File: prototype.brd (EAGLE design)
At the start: 100 x 80 mm, 15 parts

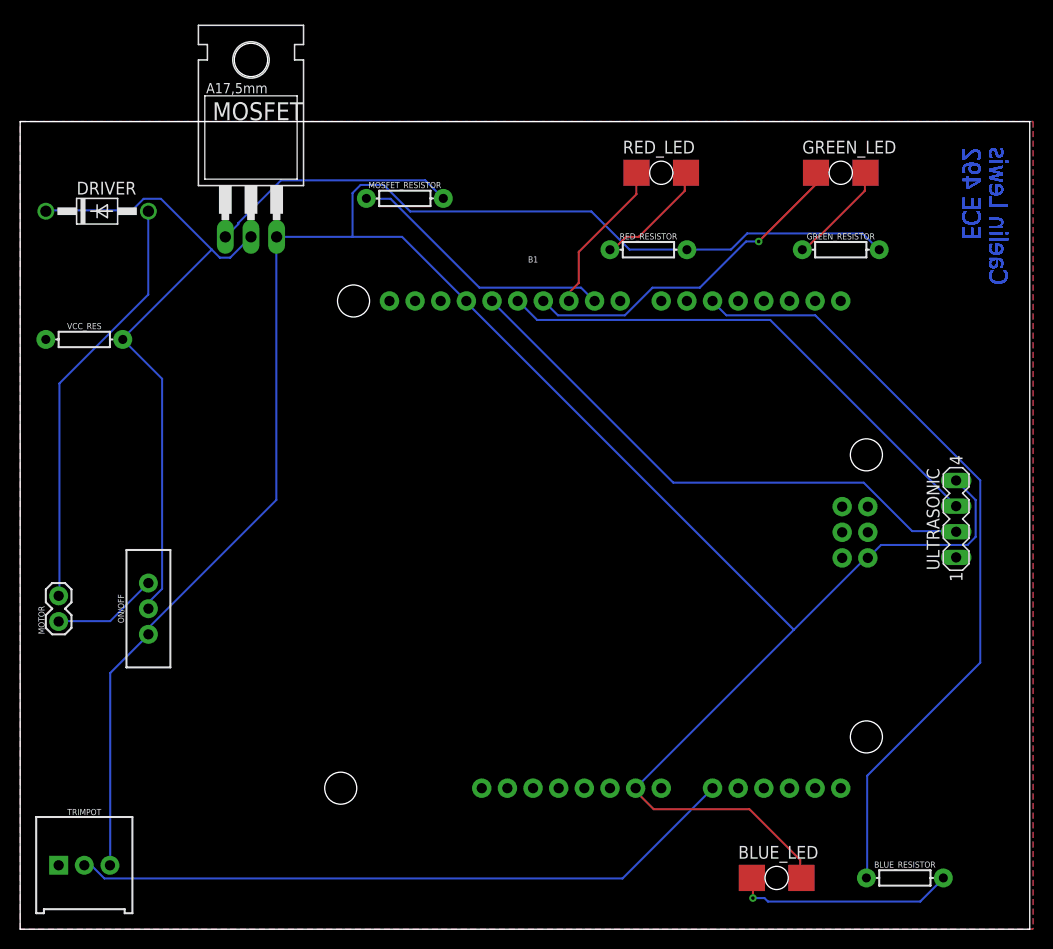
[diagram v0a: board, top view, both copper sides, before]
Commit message: Final Draft of board
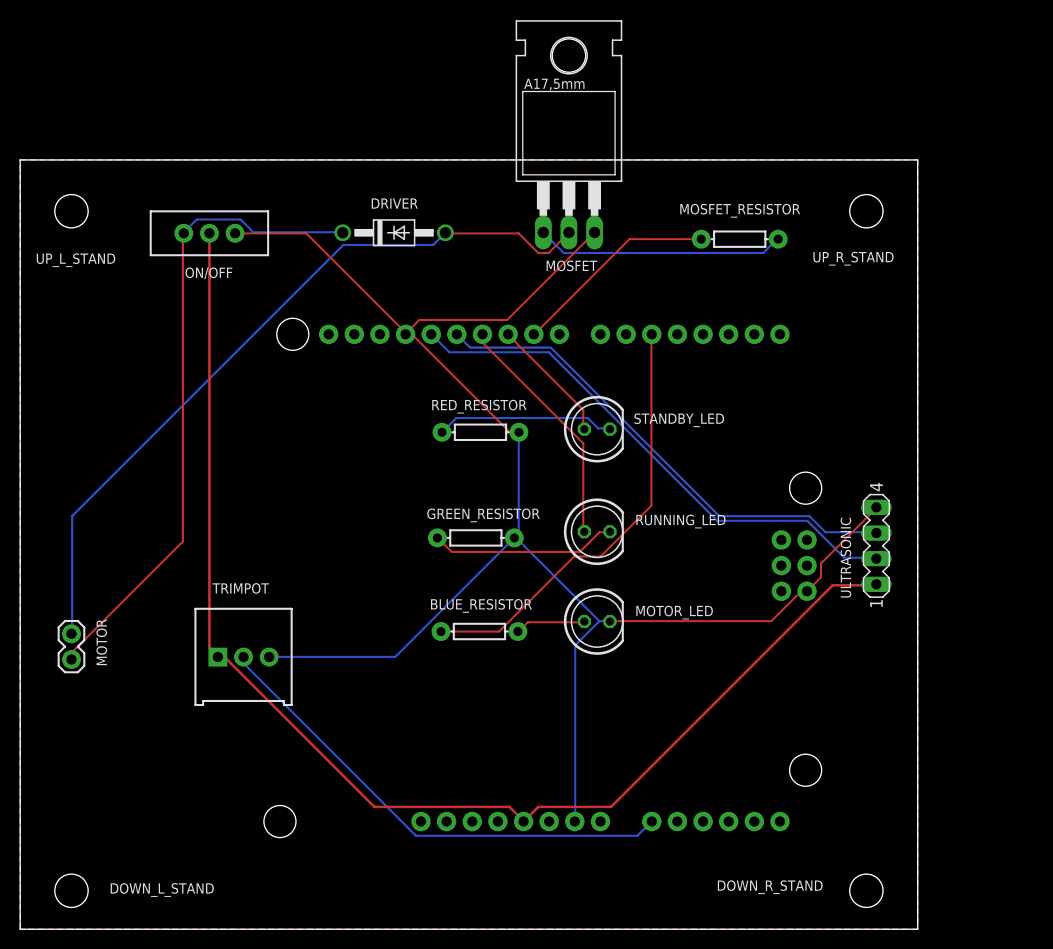
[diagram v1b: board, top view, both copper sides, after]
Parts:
- removed BLUE_LED, GREEN_LED, RED_LED: LAP4-BOTTOM, led:P47F-BOTTOM
- removed VCC_RES: 1k, SparkFun-Resistors:AXIAL-0.3
- added DOWN_L_STAND, DOWN_R_STAND, UP_L_STAND, UP_R_STAND: (no value), SparkFun-Hardware:STAND-OFF
- added MOTOR_LED: BLUE, led:LED5MM
- added RUNNING_LED: GREEN, led:LED5MM
- added STANDBY_LED: RED, led:LED5MM
- moved BLUE_RESISTOR 48.7 mm to (45.5, 29.5)
- moved GREEN_RESISTOR 46.1 mm to (45.1, 38.8)
- moved ON/OFF 37.7 mm to (18.7, 68.9), turned to 90 degrees
- moved MOSFET_RESISTOR 33.4 mm to (71.3, 68.4)
- moved MOSFET 31.5 mm to (54.4, 75.4)
- moved DRIVER 29.5 mm to (37.0, 69.0)
- moved TRIMPOT 26.0 mm to (22.1, 27.0)
- moved RED_RESISTOR 24.6 mm to (45.6, 49.2)
- moved ULTRASONIC 8.34 mm to (84.8, 38.0)
- moved B1 6.87 mm to (44.8, 34.8)
- moved MOTOR 3.97 mm to (5.08, 26.7)
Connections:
- removed net N$10: MOTOR.1, ON/OFF.1
- removed net N$11: DRIVER.A, MOTOR.2
- new net N$1: DRIVER.C, MOTOR.1, ON/OFF.1
- net GND: now also MOTOR_LED.K; no longer BLUE_LED.C
- net GREEN: now also RUNNING_LED.A; no longer GREEN_LED.A
- net N$4: now also STANDBY_LED.K; no longer RED_LED.C
- net N$5: now also RUNNING_LED.K; no longer GREEN_LED.C
- net N$8: now also MOTOR_LED.A; no longer BLUE_LED.A
- net N$9: now also DRIVER.A, MOTOR.2; no longer DRIVER.C, ON/OFF.2, VCC_RES.P$2
- net RED: now also STANDBY_LED.A; no longer RED_LED.A
- net VCC: now also ON/OFF.2; no longer VCC_RES.P$1
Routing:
- net VCC: track 0.00 -> 124.1 mm
- net GND: track 269.1 -> 165.1 mm
- net N$1: track 0.00 -> 63.8 mm
- net N$11: track 41.8 -> 0.00 mm
- net BLUE: track 78.0 -> 43.0 mm
- net POTENTIOMETER: track 66.5 -> 48.7 mm
- net N$8: track 22.1 -> 6.98 mm, vias 1 -> 0
- net N$10: track 10.5 -> 0.00 mm
- net GREEN: track 34.1 -> 23.7 mm, vias 1 -> 0
- net N$9: track 65.5 -> 74.2 mm
- net N$5: track 10.4 -> 18.5 mm
- net MOSFET: track 26.8 -> 20.5 mm
- net N$4: track 11.7 -> 17.7 mm
- net RED: track 15.5 -> 12.5 mm
- net TRIG: track 55.5 -> 53.4 mm
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- added copper zone on layer 1, net N$2
- added copper zone on layer 16, net N$3
- removed copper zone on layer 16, net GRND
- removed copper zone on layer 1, net VCC
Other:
- board size 100 x 80 mm -> 88.9 x 76.2 mm
- board text added: "ECE 492 Caelin Lewis"
- board text removed: "Caelin Lewis ECE 492"
